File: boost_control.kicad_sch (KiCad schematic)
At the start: 0 parts

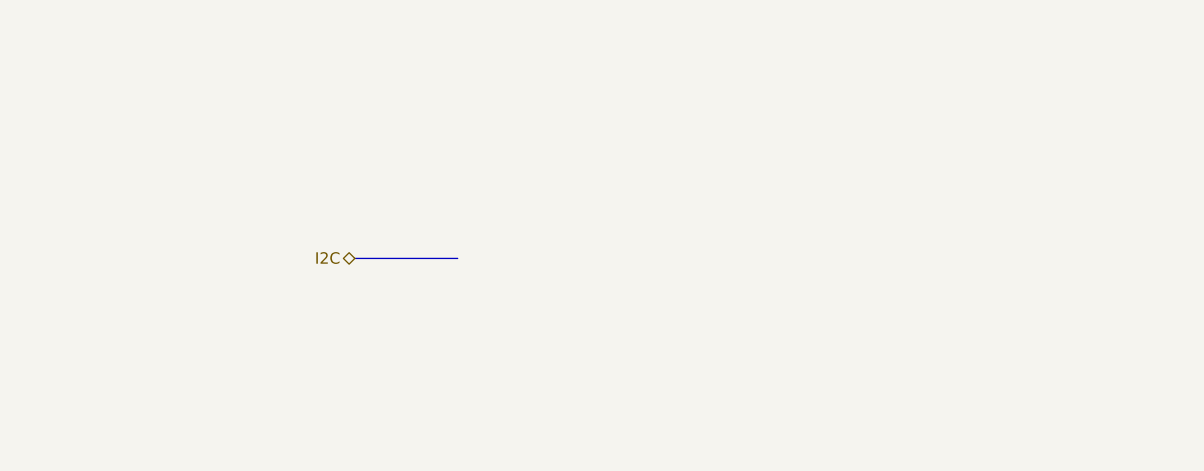
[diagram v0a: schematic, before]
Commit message: Adding control stuff
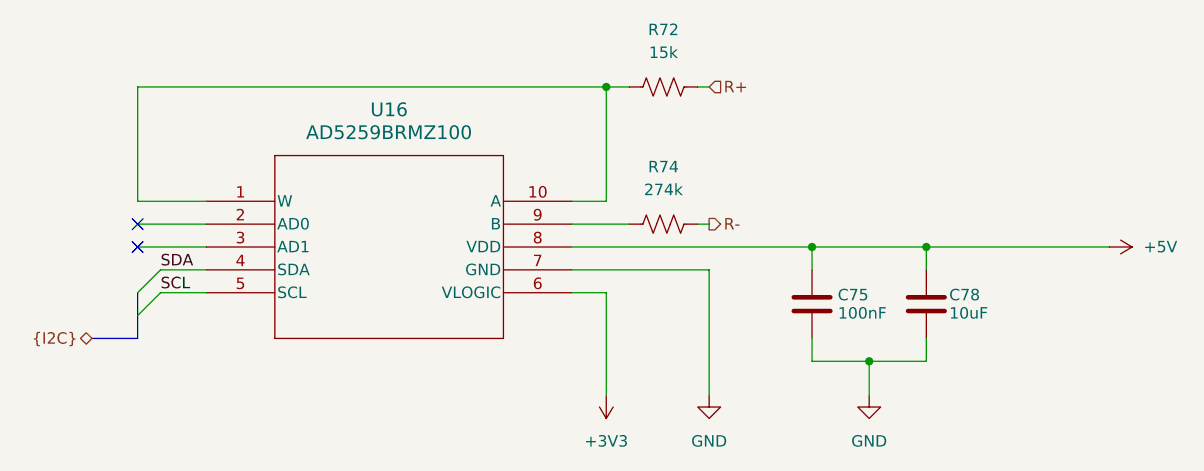
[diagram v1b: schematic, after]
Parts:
- added C75: 100nF, Capacitor_SMD:C_0603_1608Metric, symbol Device:C
- added C78: 10uF, Capacitor_SMD:C_0805_2012Metric, symbol Device:C
- added R72: 15k, Resistor_SMD:R_0603_1608Metric, symbol Device:R_US
- added R74: 274k, Resistor_SMD:R_0603_1608Metric, symbol Device:R_US
- added U16: AD5259BRMZ100, RM_10_ADI, symbol _AD5259:AD5259BRMZ100
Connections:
- new net: R72.1, U16.1 (W), U16.10 (A)
- new net: R74.1, U16.9 (B)
- new net +3V3: U16.6 (VLOGIC)
- new net +5V: C75.1, C78.1, U16.8 (VDD)
- new net GND: C75.2, C78.2, U16.7 (GND)
- new net R+: R72.2
- new net R-: R74.2
- new net SCL: U16.5 (SCL)
- new net SDA: U16.4 (SDA)
- no-connect marks 0 -> 2
